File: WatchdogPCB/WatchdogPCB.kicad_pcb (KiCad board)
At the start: 2 copper layers, 5 parts, among them J1 Conn_01x05_Socket, J2 Conn_01x05_Pin, J3 Screw_Terminal_01x03, J4 Power

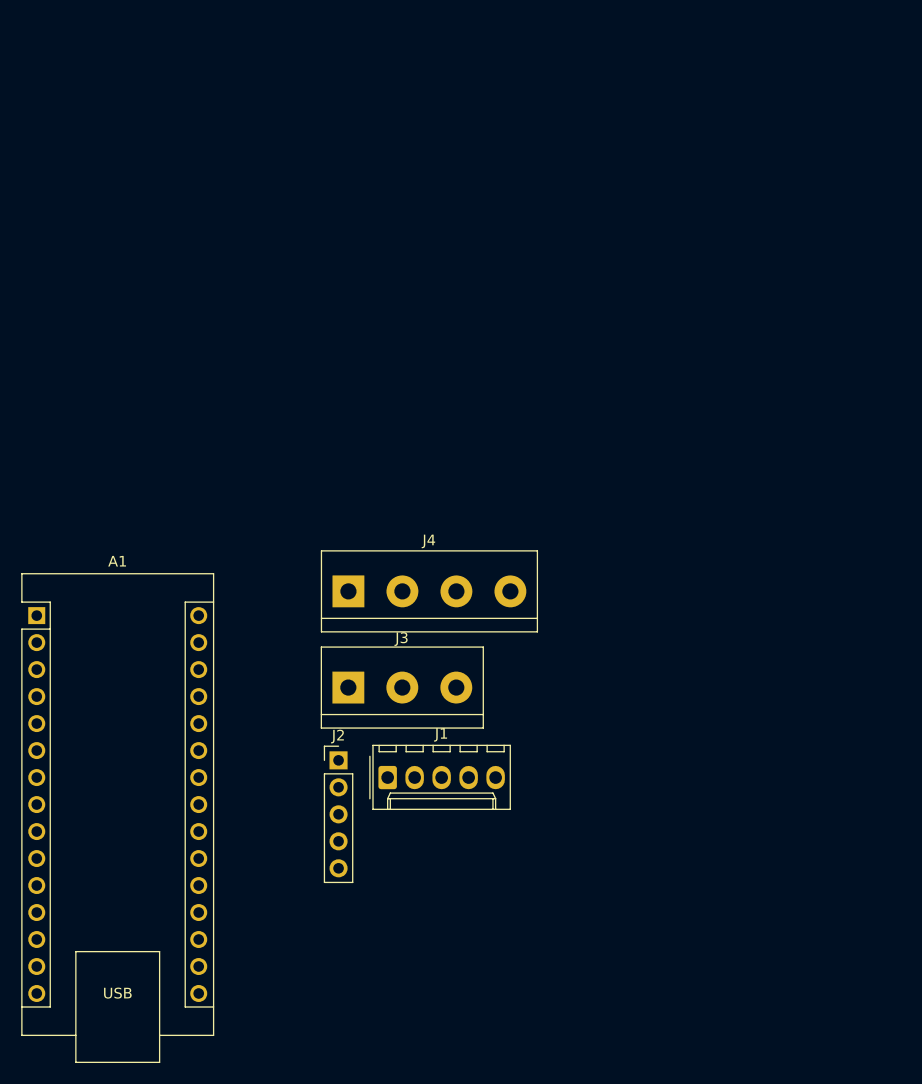
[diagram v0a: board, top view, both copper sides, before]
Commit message: Layout mostly done
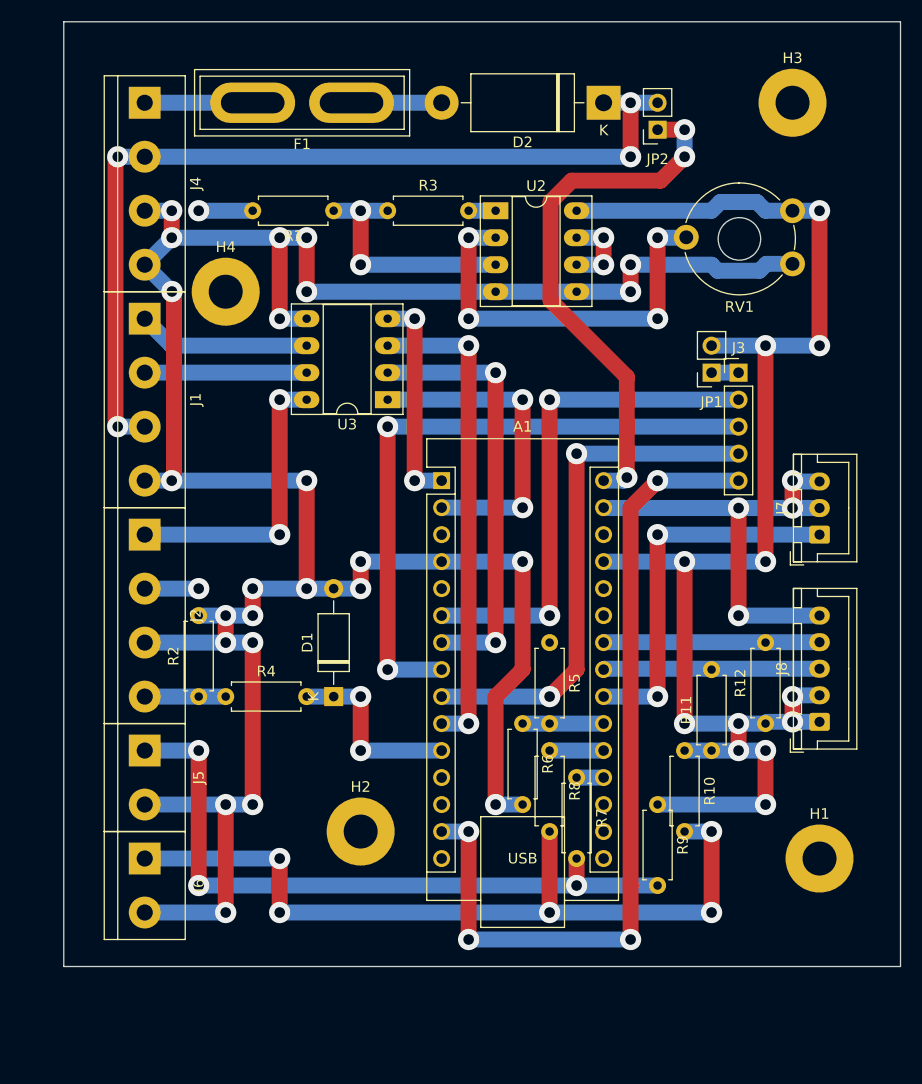
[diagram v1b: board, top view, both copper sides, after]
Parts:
- added D1: 5.1V, Diode_THT:D_A-405_P10.16mm_Horizontal, F.Cu at (101.6, 94.0)
- added D2: 1N5404, Diode_THT:D_DO-201AD_P15.24mm_Horizontal, F.Cu at (127.0, 38.1)
- added F1: 3A, Fuse:Fuse_Blade_ATO_directSolder, F.Cu at (103.3, 38.1)
- added H1: MountingHole, MountingHole:MountingHole_3.2mm_M3_Pad, F.Cu at (147.3, 109.2)
- added H2: MountingHole, MountingHole:MountingHole_3.2mm_M3_Pad, F.Cu at (104.1, 106.7)
- added H3: MountingHole, MountingHole:MountingHole_3.2mm_M3_Pad, F.Cu at (144.8, 38.1)
- added H4: MountingHole, MountingHole:MountingHole_3.2mm_M3_Pad, F.Cu at (91.4, 55.9)
- added J5: Thermistor 1, TerminalBlock:TerminalBlock_bornier-2_P5.08mm, F.Cu at (83.8, 99.1)
- added J6: Thermistor 2, TerminalBlock:TerminalBlock_bornier-2_P5.08mm, F.Cu at (83.8, 109.2)
- added J7: Dashboard A, Connector_JST:JST_XH_B3B-XH-A_1x03_P2.50mm_Vertical, F.Cu at (147.3, 78.7)
- added J8: Dashboard B, Connector_JST:JST_XH_B5B-XH-A_1x05_P2.50mm_Vertical, F.Cu at (147.3, 96.4)
- added JP1: 5V jumper, Connector_PinSocket_2.54mm:PinSocket_1x02_P2.54mm_Vertical, F.Cu at (137.2, 63.5)
- added JP2: 12V jumper, Connector_PinSocket_2.54mm:PinSocket_1x02_P2.54mm_Vertical, F.Cu at (132.1, 40.6)
- added R1: 4.7k, Resistor_THT:R_Axial_DIN0207_L6.3mm_D2.5mm_P7.62mm_Horizontal, F.Cu at (101.6, 48.3)
- added R10: 470, Resistor_THT:R_Axial_DIN0207_L6.3mm_D2.5mm_P7.62mm_Horizontal, F.Cu at (134.6, 99.1)
- added R11: 4.7k, Resistor_THT:R_Axial_DIN0207_L6.3mm_D2.5mm_P7.62mm_Horizontal, F.Cu at (137.2, 99.1)
- added R12: 4.7k, Resistor_THT:R_Axial_DIN0207_L6.3mm_D2.5mm_P7.62mm_Horizontal, F.Cu at (142.2, 96.5)
- added R2: 1k, Resistor_THT:R_Axial_DIN0207_L6.3mm_D2.5mm_P7.62mm_Horizontal, F.Cu at (88.9, 94.0)
- added R3: 120k, Resistor_THT:R_Axial_DIN0207_L6.3mm_D2.5mm_P7.62mm_Horizontal, F.Cu at (106.7, 48.3)
- added R4: 4.7k, Resistor_THT:R_Axial_DIN0207_L6.3mm_D2.5mm_P7.62mm_Horizontal, F.Cu at (91.4, 94.0)
- added R5: 100k, Resistor_THT:R_Axial_DIN0207_L6.3mm_D2.5mm_P7.62mm_Horizontal, F.Cu at (121.9, 88.9)
- added R6: 39k, Resistor_THT:R_Axial_DIN0207_L6.3mm_D2.5mm_P7.62mm_Horizontal, F.Cu at (119.4, 96.5)
- added R7: 1k, Resistor_THT:R_Axial_DIN0207_L6.3mm_D2.5mm_P7.62mm_Horizontal, F.Cu at (124.5, 101.6)
- added R8: 1k, Resistor_THT:R_Axial_DIN0207_L6.3mm_D2.5mm_P7.62mm_Horizontal, F.Cu at (121.9, 99.1)
- added R9: 470, Resistor_THT:R_Axial_DIN0207_L6.3mm_D2.5mm_P7.62mm_Horizontal, F.Cu at (132.1, 104.1)
- added RV1: 10k, Potentiometer_THT:Potentiometer_Piher_PT-10-V10_Vertical_Hole, F.Cu at (144.8, 48.3)
- added U2: MCP602, Package_DIP:DIP-8_W7.62mm_Socket_LongPads, F.Cu at (116.8, 48.3)
- added U3: DS3695N, Package_DIP:DIP-8_W7.62mm_Socket_LongPads, F.Cu at (106.7, 66.0)
- J1: value Conn_01x05_Socket -> Roll hoop; footprint Connector_Molex:Molex_KK-254_AE-6410-05A_1x05_P2.54mm_Vertical -> TerminalBlock:TerminalBlock_bornier-4_P5.08mm
- J2: value Conn_01x05_Pin -> Speed & Oil; footprint Connector_PinHeader_2.54mm:PinHeader_1x05_P2.54mm_Vertical -> TerminalBlock:TerminalBlock_bornier-4_P5.08mm
- J3: value Screw_Terminal_01x03 -> H bridge driver control; footprint TerminalBlock:TerminalBlock_bornier-3_P5.08mm -> Connector_PinHeader_2.54mm:PinHeader_1x05_P2.54mm_Vertical
- moved J4 49.8 mm to (83.8, 38.1), turned to -90 degrees
- moved J1 48.9 mm to (83.8, 58.4), turned to -90 degrees
- moved J3 47.2 mm to (139.7, 63.5)
- moved A1 40.2 mm to (111.8, 73.7)
- moved J2 28.0 mm to (83.8, 78.7), turned to -90 degrees
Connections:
- A1 pad 1: unconnected-(A1-D1/TX-Pad1) -> Net-(A1-D1/TX)
- A1 pad 10: unconnected-(A1-D7-Pad10) -> Net-(A1-D7)
- A1 pad 11: unconnected-(A1-D8-Pad11) -> Net-(A1-D8)
- A1 pad 14: unconnected-(A1-D11-Pad14) -> Net-(A1-D11)
- A1 pad 19: unconnected-(A1-A0-Pad19) -> Net-(A1-A0)
- A1 pad 2: unconnected-(A1-D0/RX-Pad2) -> Net-(A1-D0/RX)
- A1 pad 20: unconnected-(A1-A1-Pad20) -> Net-(A1-A1)
- A1 pad 21: unconnected-(A1-A2-Pad21) -> Net-(A1-A2)
- A1 pad 22: unconnected-(A1-A3-Pad22) -> /Button
- A1 pad 23: unconnected-(A1-A4-Pad23) -> /SDA
- A1 pad 24: unconnected-(A1-A5-Pad24) -> /SCL
- A1 pad 27: unconnected-(A1-+5V-Pad27) -> +5V
- A1 pad 29: unconnected-(A1-GND-Pad29) -> GND
- A1 pad 30: unconnected-(A1-VIN-Pad30) -> Net-(A1-VIN)
- A1 pad 4: unconnected-(A1-GND-Pad4) -> GND
- A1 pad 5: unconnected-(A1-D2-Pad5) -> Net-(A1-D2)
- A1 pad 6: unconnected-(A1-D3-Pad6) -> Net-(A1-D3)
- A1 pad 7: unconnected-(A1-D4-Pad7) -> Net-(A1-D4)
- A1 pad 8: unconnected-(A1-D5-Pad8) -> Net-(A1-D5)
- A1 pad 9: unconnected-(A1-D6-Pad9) -> Net-(A1-D6)
- J1 pad 1: unconnected-(J1-Pin_1-Pad1) -> Net-(J1-Pin_1)
- J1 pad 2: unconnected-(J1-Pin_2-Pad2) -> Net-(J1-Pin_2)
- J1 pad 3: unconnected-(J1-Pin_3-Pad3) -> +12V
- J1 pad 4: unconnected-(J1-Pin_4-Pad4) -> GND
- J2 pad 1: unconnected-(J2-Pin_1-Pad1) -> +5V
- J2 pad 2: unconnected-(J2-Pin_2-Pad2) -> /Hall effect
- J2 pad 3: unconnected-(J2-Pin_3-Pad3) -> GND
- J2 pad 4: unconnected-(J2-Pin_4-Pad4) -> /Oil
- J3 pad 1: unconnected-(J3-Pin_1-Pad1) -> Net-(J3-Pin_1)
- J3 pad 2: unconnected-(J3-Pin_2-Pad2) -> Net-(A1-D3)
- J3 pad 3: unconnected-(J3-Pin_3-Pad3) -> Net-(A1-D5)
- J4 pad 1: Net-(J4-Pin_1) -> /Power in
- J4 pad 2: Net-(J4-Pin_2) -> +12V
- J4 pad 3: Net-(J4-Pin_1) -> GND
- J4 pad 4: Net-(J4-Pin_2) -> GND
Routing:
- net GND: track 0.00 -> 303.2 mm, vias 0 -> 28
- net +5V: track 0.00 -> 209.4 mm, vias 0 -> 14
- net +12V: track 0.00 -> 86.5 mm, vias 0 -> 4
- net Net-(A1-D11): track 0.00 -> 79.8 mm, vias 0 -> 4
- net Net-(J6-Pin_1): track 0.00 -> 76.2 mm, vias 0 -> 5
- net +BATT: track 0.00 -> 67.9 mm
- net Net-(J5-Pin_1): track 0.00 -> 63.5 mm, vias 0 -> 3
- net Net-(A1-D5): track 0.00 -> 61.0 mm, vias 0 -> 2
- net /Hall effect: track 0.00 -> 59.6 mm, vias 0 -> 2
- net Net-(A1-VIN): track 0.00 -> 50.7 mm, vias 0 -> 3
- net Net-(A1-D6): track 0.00 -> 49.3 mm, vias 0 -> 2
- net Net-(A1-D3): track 0.00 -> 48.3 mm, vias 0 -> 2
- net Net-(A1-D2): track 0.00 -> 46.3 mm
- net Net-(A1-D7): track 0.00 -> 45.7 mm, vias 0 -> 2
- net Net-(A1-D4): track 0.00 -> 40.6 mm, vias 0 -> 2
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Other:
- board outline added: 78.7 x 88.9 mm
- copper layers 2 -> 4
